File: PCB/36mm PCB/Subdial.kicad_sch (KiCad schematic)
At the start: 9 parts, among them Q3 2N7002KQBZ, Q4 2N7002KQBZ, Q5 2N7002KQBZ, Q6 2N7002KQBZ

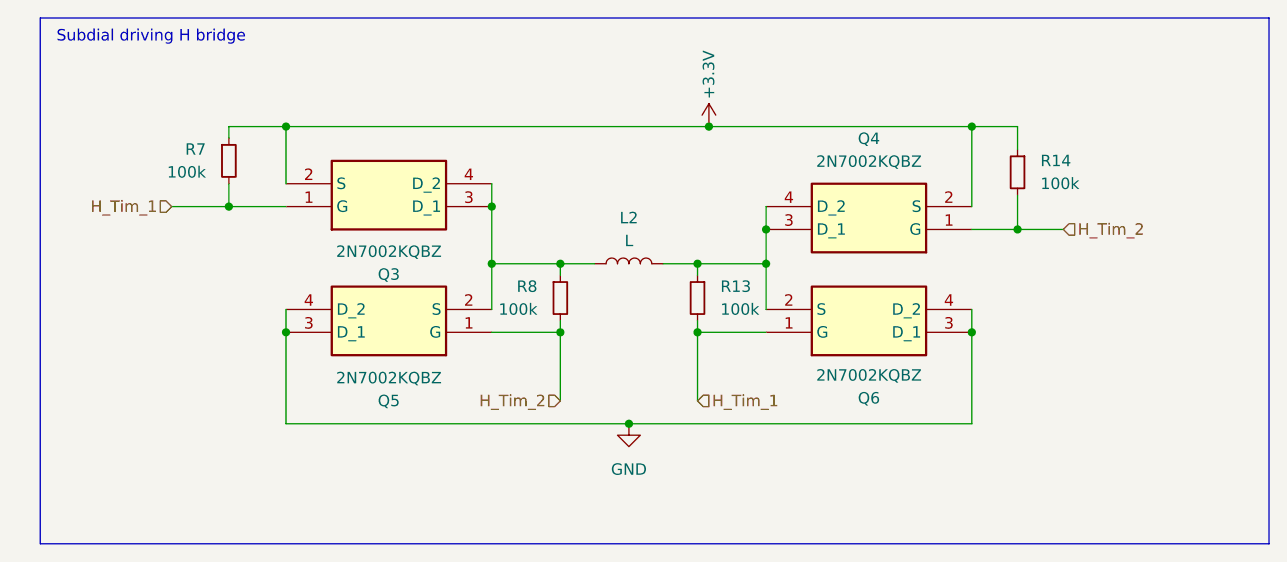
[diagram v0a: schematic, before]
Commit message: Modifs Mathieu
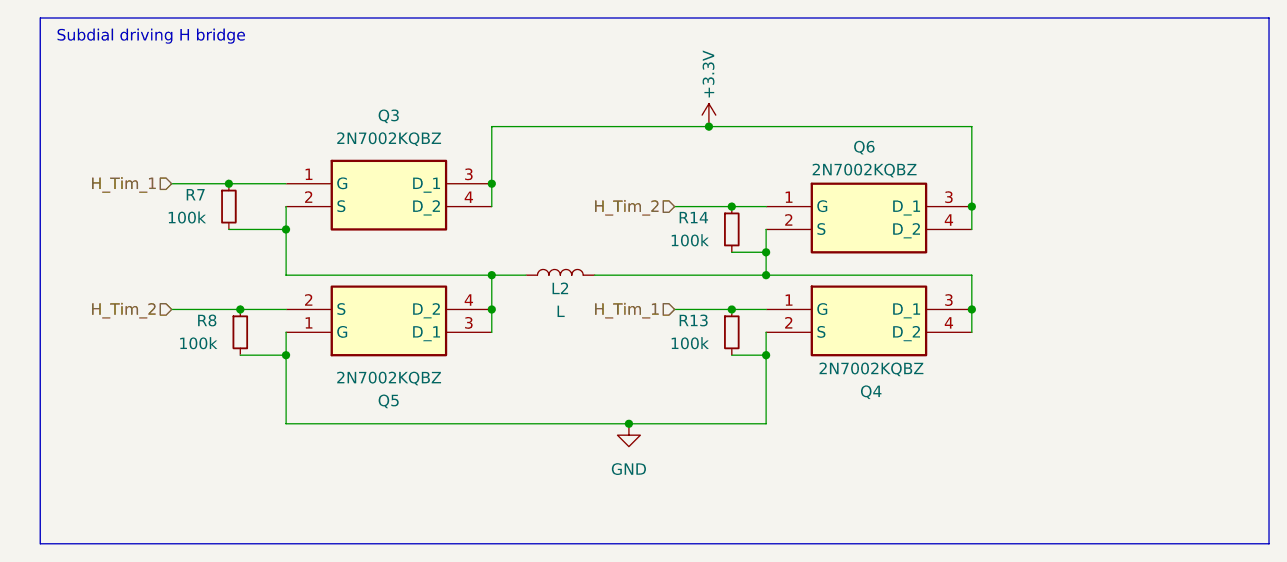
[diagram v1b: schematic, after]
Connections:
- net +3.3V: now also Q3.3 (D_1), Q3.4 (D_2), Q4.3 (D_1), Q4.4 (D_2); no longer Q3.2 (S), Q4.2 (S), R14.1, R7.1
- net GND: now also Q5.1 (G), Q6.2 (S), R13.2, R8.2; no longer Q5.3 (D_1), Q5.4 (D_2), Q6.3 (D_1), Q6.4 (D_2)
- net H_Tim_1: now also R13.1, R7.1; no longer R13.2, R7.2
- net H_Tim_2: now also Q5.2 (S), R14.1, R8.1; no longer Q5.1 (G), R14.2, R8.2
- new net: L2.2, Q4.2 (S), Q6.3 (D_1), Q6.4 (D_2), R14.2
- new net: L2.1, Q3.2 (S), Q5.3 (D_1), Q5.4 (D_2), R7.2
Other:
- moved on the sheet: L2, Q4, Q5, R13, R14, R7, R8
